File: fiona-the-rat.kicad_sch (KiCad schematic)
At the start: 65 parts, among them J1 USB_TP_P, J10 ~{CHG}_TP, J11 +1V1_TP, J12 VBAT_TP, J13 +3V3_TP, J14 SWD, J19 GPIO0, J2 USB_TP_N, J20 GPIO1, J21 GPIO2, J22 Haptics, J3 XTAL_TP, J4 USB_C_Receptacle_PowerOnly_6P, J5 VBAT_ADC_TP, J6 Periph, J7 GND_TP_1, J8 GND_TP_2, J9 GND_TP_3, Q1 MMBT2222A, SW1 1825027-8, U1 RP2040, U3 W25Q128JVSIQ, U4 BQ21040DBVR, U5 AP2112K-3.3, Y1 Crystal_GND24

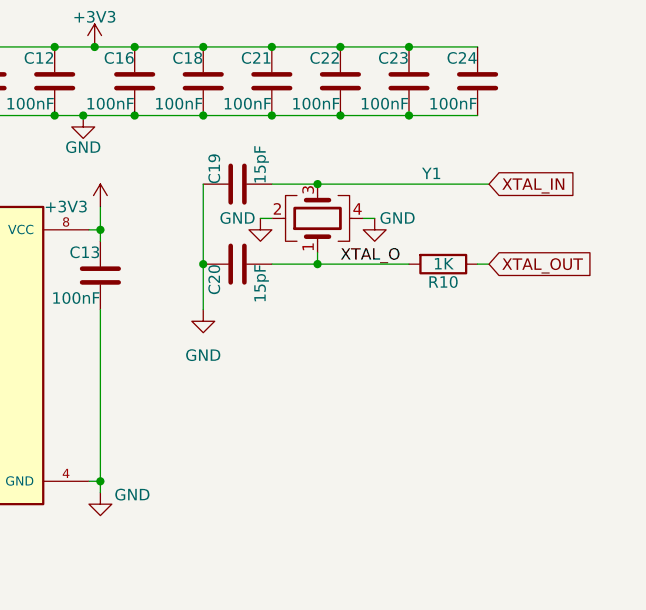
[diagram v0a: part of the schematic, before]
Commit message: swap crystal lib
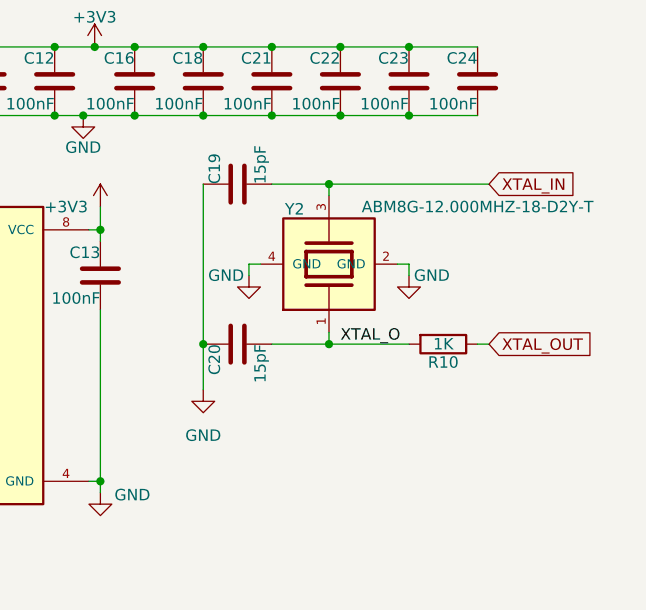
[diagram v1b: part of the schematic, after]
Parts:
- removed Y1: Crystal_GND24, Crystal:Crystal_SMD_Abracon_ABM8G-4Pin_3.2x2.5mm, symbol Device:Crystal_GND24
- added Y2: ABM8G-12.000MHZ-18-D2Y-T, pfornage-kicad-lib:XTAL_ABM8G-12.000MHZ-18-D2Y-T, symbol pfornage-kicad-lib:ABM8G-12.000MHZ-18-D2Y-T
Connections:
- net GND: now also Y2.2 (GND), Y2.4 (GND)
- net XTAL_IN: now also Y2.3
- net XTAL_O: now also Y2.1
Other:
- moved on the sheet: C20, R10
